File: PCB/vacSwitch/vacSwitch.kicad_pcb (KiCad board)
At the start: 2 copper layers, 91.2 x 50.8 mm, 28 parts, among them J1 Mains, J2 RS232, J3 ISP, J4 VoltFreeContact, K1 HE721A0510, Q1 BC547, U1 ATtiny85-20PU, U2 ACS712xLCTR-20A, U3 MOC3043M

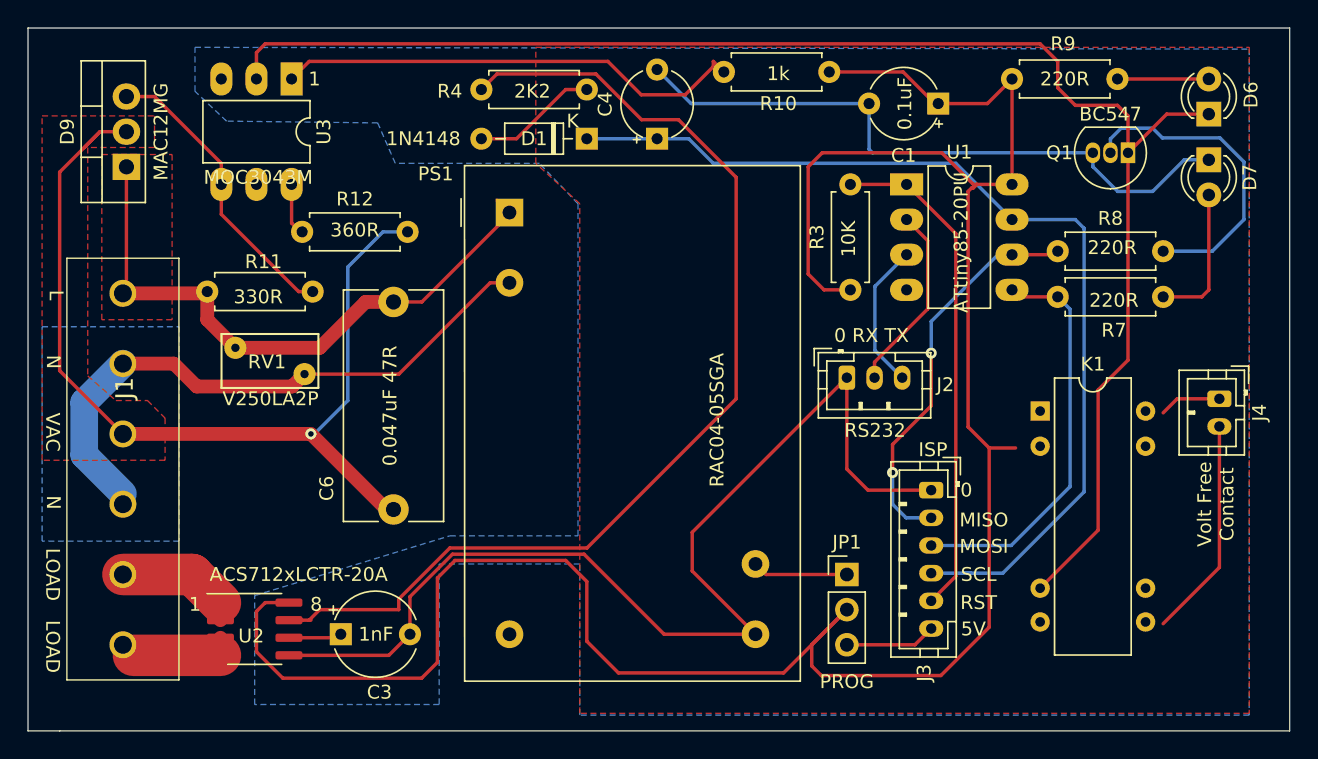
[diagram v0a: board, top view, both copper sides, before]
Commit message: Defaults tweak
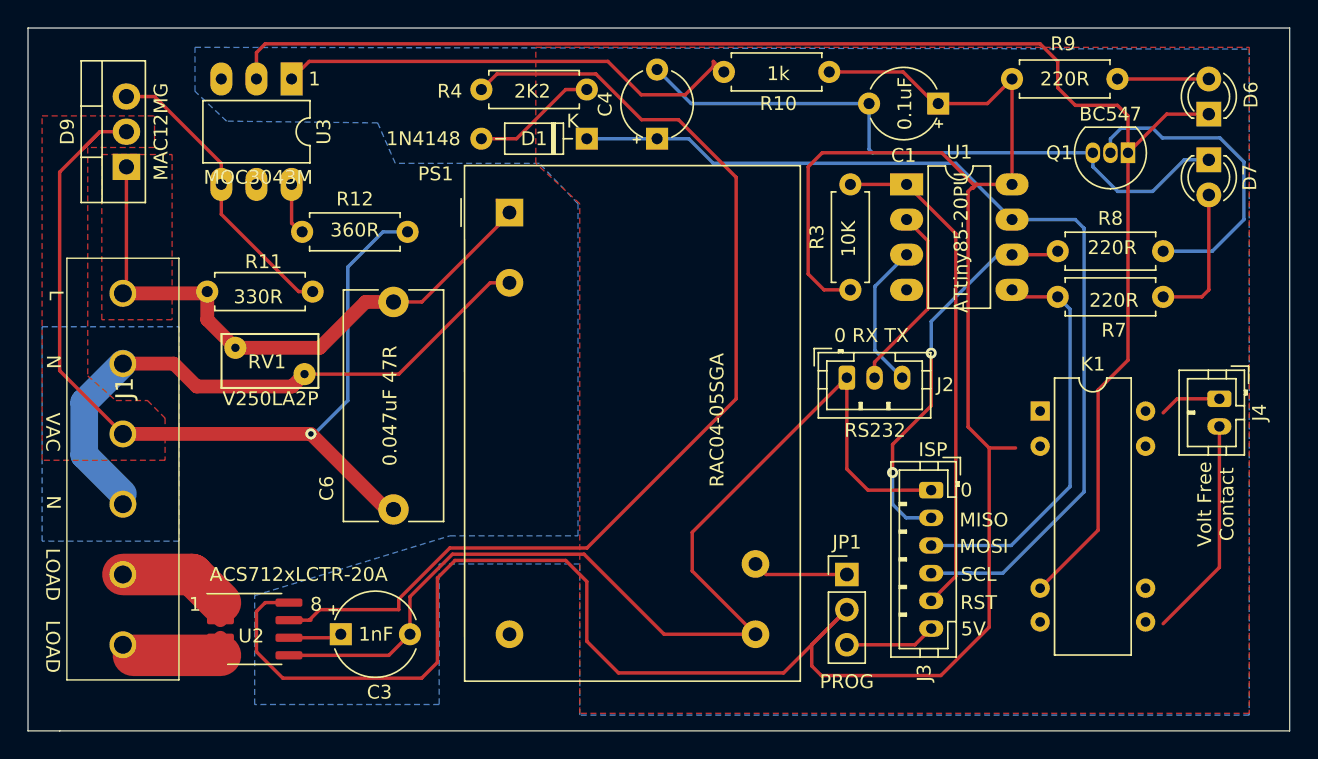
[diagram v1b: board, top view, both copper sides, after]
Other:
- net class Default removed
